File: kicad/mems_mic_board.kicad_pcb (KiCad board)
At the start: 2 copper layers, 9 parts, among them J1 Conn_01x06_Male, J2 Conn_01x01_Male, J3 Conn_01x06_Male, J4 Conn_01x06_Female, J6 Conn_01x08_Male, J7 Conn_01x08_Male, U1 tactile_sw, U2 mems_mic, U3 mems_mic

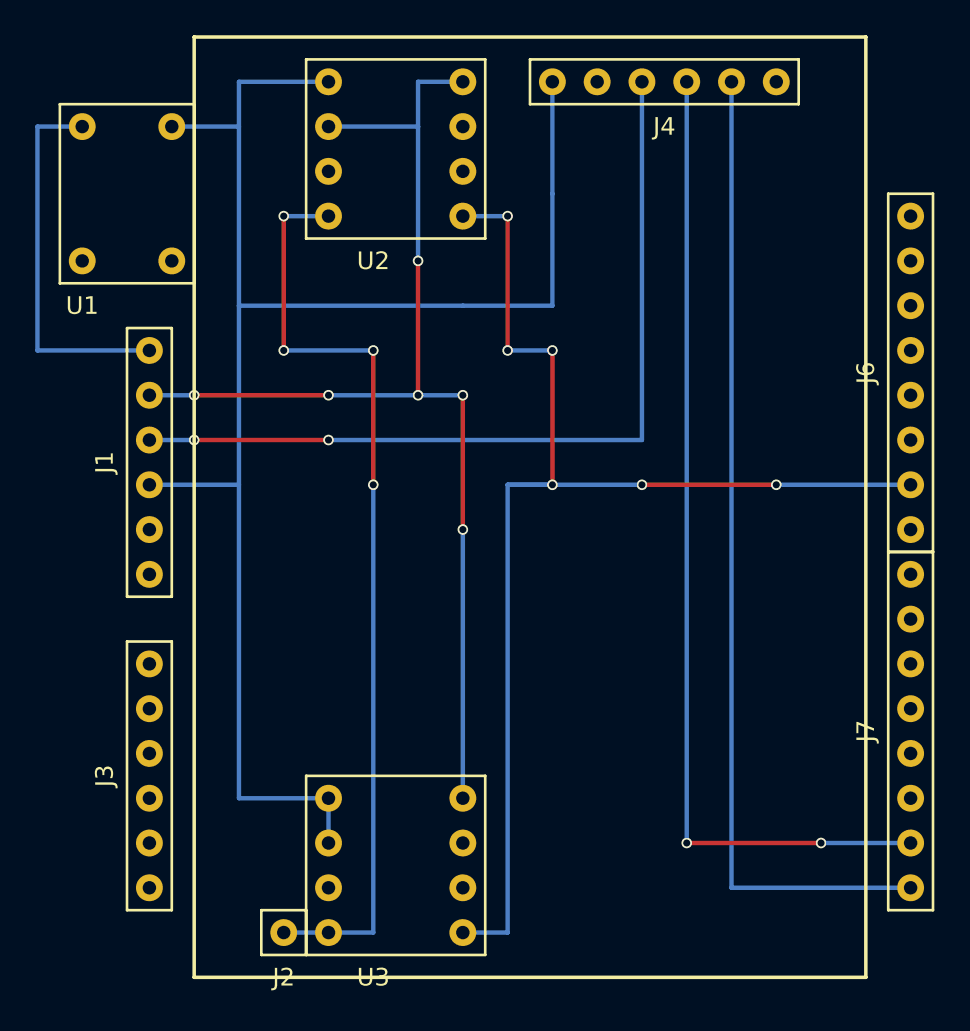
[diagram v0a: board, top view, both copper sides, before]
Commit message: update
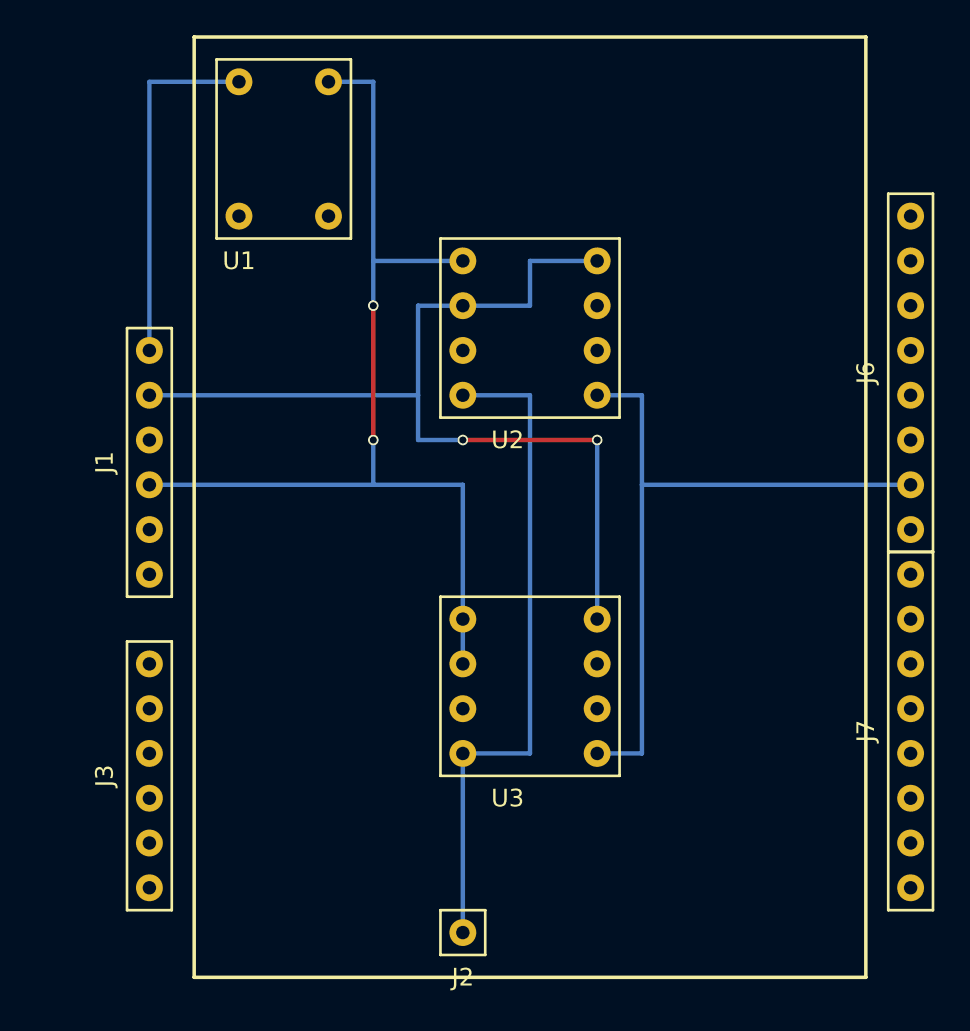
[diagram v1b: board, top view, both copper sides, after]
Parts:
- removed J4: Conn_01x06_Female, mcu:Pin Header 6P
- moved U3 12.7 mm to (133.3, 121.9)
- moved U2 12.7 mm to (133.3, 101.6)
- moved J2 10.2 mm to (129.5, 135.9)
- moved U1 9.25 mm to (119.4, 91.4)
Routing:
- net Net-(J4-Pad5): track 55.9 -> 0.00 mm
- net Net-(J4-Pad4): track 55.9 -> 0.00 mm, vias 2 -> 0
- net Net-(J1-Pad3): track 48.3 -> 0.00 mm, vias 2 -> 0
- net GND: track 92.7 -> 58.4 mm, vias 0 -> 2
- net Net-(J6-Pad7): track 73.7 -> 40.6 mm, vias 6 -> 0
- net Net-(J2-Pad1): track 53.3 -> 38.1 mm, vias 4 -> 0
- net +3V3: track 66.0 -> 55.9 mm, vias 6 -> 2
- net Net-(J1-Pad1): track 21.6 -> 20.3 mm
